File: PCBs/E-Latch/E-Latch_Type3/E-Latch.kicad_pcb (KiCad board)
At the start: 2 copper layers, 43.2 x 68.6 mm, 17 parts, among them J1 POWER, J2 SIG, J3 MOTOR, K1 G5LE-1, K2 G5LE-1, K3 G5LE-1, U1 LM1117-3.3

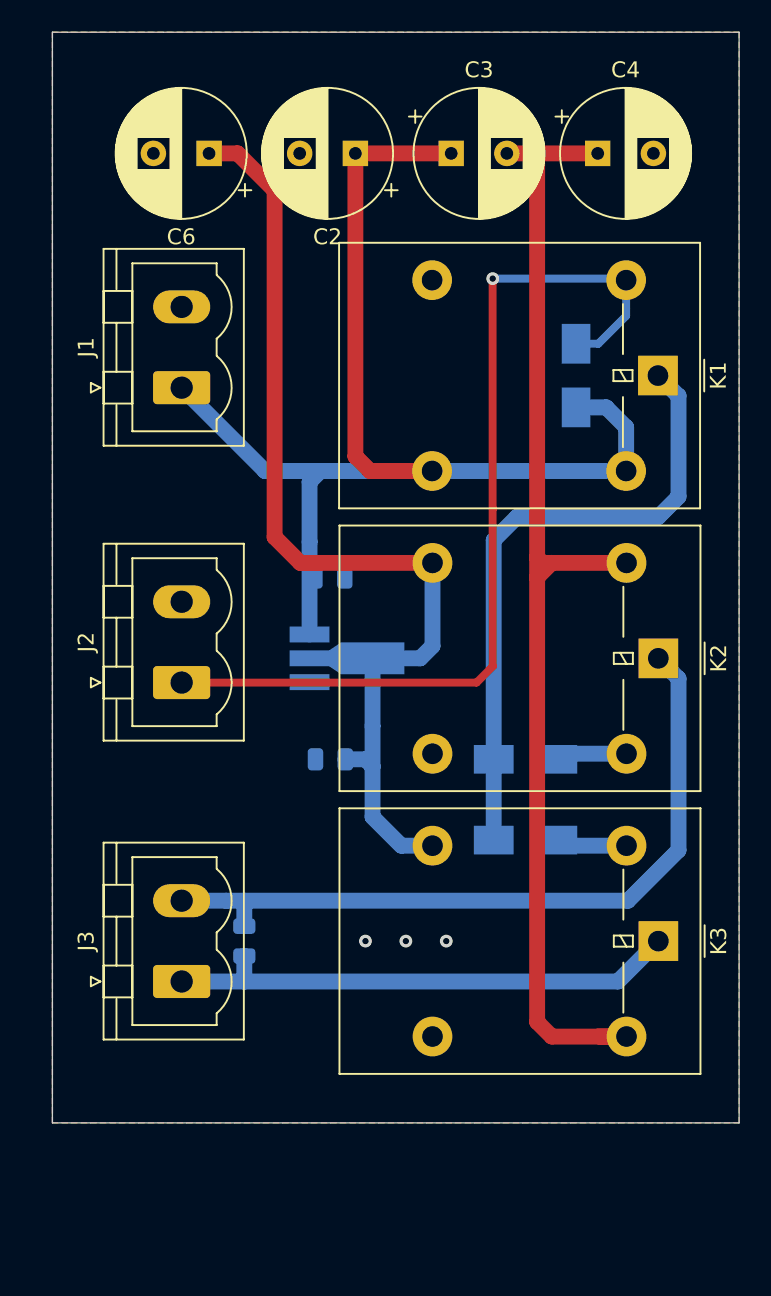
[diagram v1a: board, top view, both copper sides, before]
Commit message: Update ts when open file
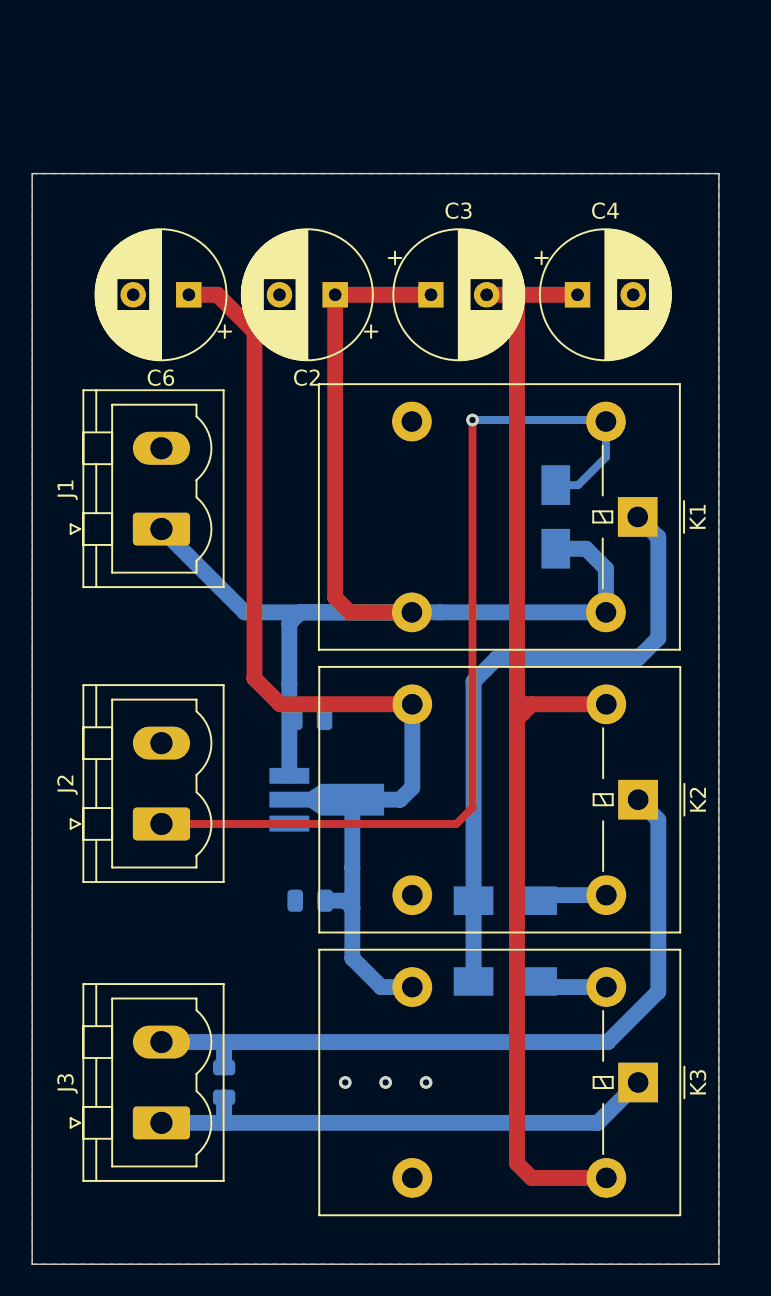
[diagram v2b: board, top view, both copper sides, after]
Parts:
- moved C2 8.98 mm to (101.6, 71.1)
- moved C3 8.98 mm to (107.6, 71.1)
- moved C4 8.98 mm to (116.8, 71.1)
- moved C6 8.98 mm to (92.4, 71.1)
- moved C7 8.98 mm to (94.6, 120.7)
- moved D3 8.98 mm to (115.5, 85.1)
- moved C1 8.98 mm to (100.0, 97.8)
- moved C5 8.98 mm to (100.0, 109.2)
- moved D1 8.98 mm to (112.3, 109.2)
- moved D2 8.98 mm to (112.3, 114.3)
- moved J1 8.98 mm to (90.7, 85.9)
- moved J2 8.98 mm to (90.7, 104.4)
- moved J3 8.98 mm to (90.7, 123.2)
- moved K1 8.98 mm to (120.6, 85.1)
- moved K2 8.98 mm to (120.7, 102.9)
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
